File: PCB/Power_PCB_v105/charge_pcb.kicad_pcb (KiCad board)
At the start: 2 copper layers, 129.5 x 66 mm, 48 parts, among them J1 Main_PCB2, J10 Mot_Left, J11 DC/DC1, J12 DC/DC2, J2 Battery, J3 Power Switch, J4 Mow3, J5 Main_PCB1, J6 Mow2, J7 Mow1, J8 Start, J9 Mot_Right, Q1 BC547C, Q2 IRF9540N, Q3 BC547C, Q4 IRF9540N, U1 INA226, U2 INA226, U3 INA226, U4 INA226, U5 INA226, U6 INA226

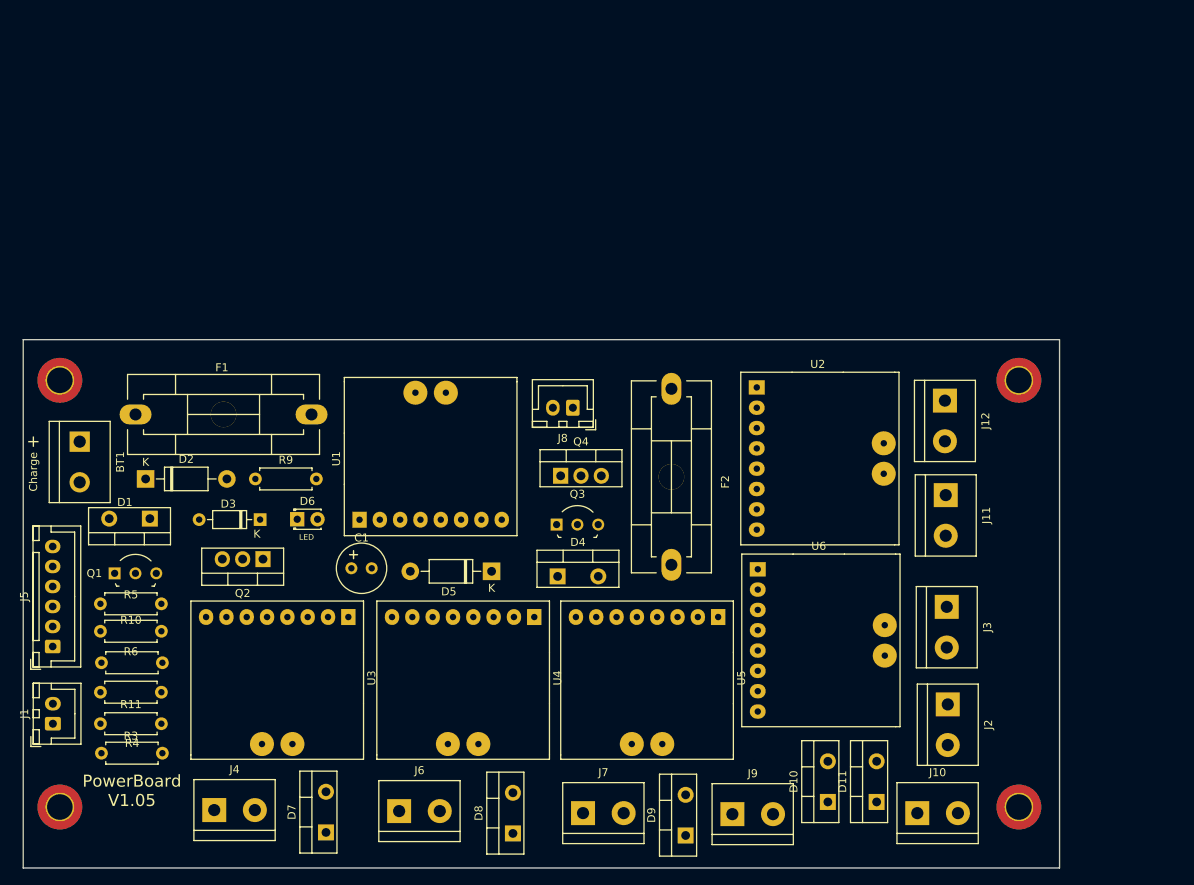
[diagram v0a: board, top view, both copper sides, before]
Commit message: power route
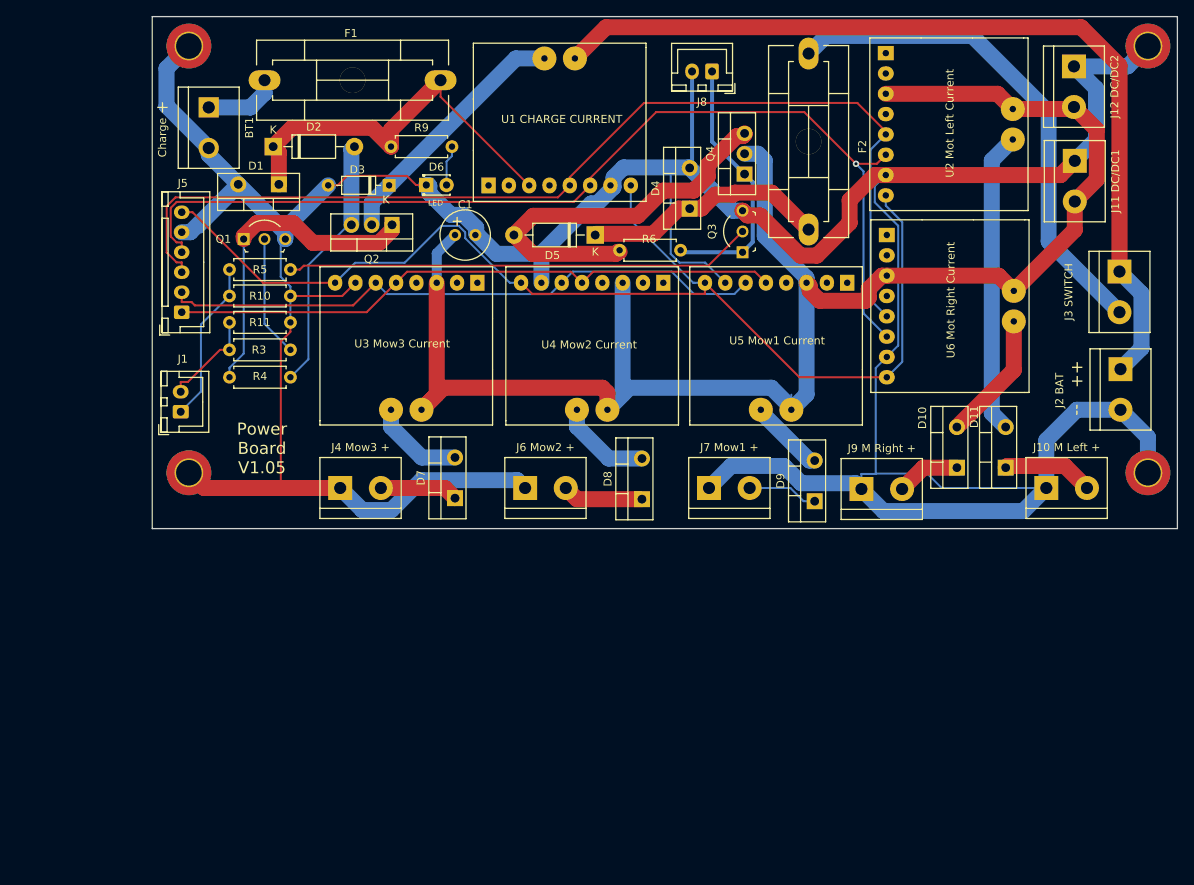
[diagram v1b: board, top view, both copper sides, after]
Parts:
- J10 M Left +: renamed from J10
- J11 DC/DC1: renamed from J11
- J12 DC/DC2: renamed from J12
- J2 BAT: renamed from J2
- J3 SWITCH: renamed from J3
- J4 Mow3 +: renamed from J4
- J6 Mow2 +: renamed from J6
- J7 Mow1 +: renamed from J7
- J9 M Right +: renamed from J9
- U1 CHARGE CURRENT: renamed from U1
- U2 Mot Left Current: renamed from U2
- U3 Mow3 Current: renamed from U3
- U4 Mow2 Current: renamed from U4
- U5 Mow1 Current: renamed from U5
- U6 Mot Right Current: renamed from U6
- moved R6 82.8 mm to (143.1, 90.4)
- moved R4 49.6 mm to (102.0, 106.3)
- moved R3 49.4 mm to (102.0, 102.9)
- moved R11 49.0 mm to (94.4, 99.4)
- moved D4 48.8 mm to (151.9, 85.2), turned to 90 degrees
- moved J2 BAT 47.1 mm to (205.7, 105.3)
- moved J3 SWITCH 47.1 mm to (205.6, 93.1)
- moved J8 45.5 mm to (154.7, 68.1)
- moved F2 45.3 mm to (166.8, 76.8)
- moved R10 44.9 mm to (94.4, 96.1)
- moved R9 44.9 mm to (114.6, 77.5)
- moved H3 44.8 mm to (209.2, 118.2)
- moved H4 44.8 mm to (89.3, 118.2)
- moved Q2 44.8 mm to (114.7, 87.2)
- moved H2 44.8 mm to (209.2, 64.9)
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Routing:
- net GND: track 0.00 -> 522.1 mm
- net V_Bat: track 0.00 -> 214.1 mm
- net +3V3: track 0.00 -> 146.2 mm
- net SCL0: track 0.00 -> 131.5 mm
- net SDA0: track 0.00 -> 127.8 mm, vias 0 -> 1
- net Net-(J2-Pad1): track 0.00 -> 111.8 mm
- net SCL1: track 0.00 -> 76.8 mm
- net SDA1: track 0.00 -> 76.5 mm
- net Net-(F2-Pad1): track 0.00 -> 63.5 mm
- net Net-(Q3-Pad2): track 0.00 -> 58.5 mm
- net V_Charge: track 0.00 -> 50.8 mm
- net Net-(D5-Pad2): track 0.00 -> 50.8 mm
- net Net-(D2-Pad2): track 0.00 -> 42.4 mm
- net Net-(Q1-Pad1): track 0.00 -> 39.9 mm
- net Net-(D11-Pad2): track 0.00 -> 37.7 mm
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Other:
- board size 129.5 x 66 mm -> 128.1 x 64 mm
- board text added: "++"
- board text added: "--"
- board text added: "Power Board V1.05"
- board text removed: "PowerBoard V1.05"
